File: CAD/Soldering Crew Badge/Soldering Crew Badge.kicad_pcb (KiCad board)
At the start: 2 copper layers, 75.2 x 75.2 mm, 7 parts

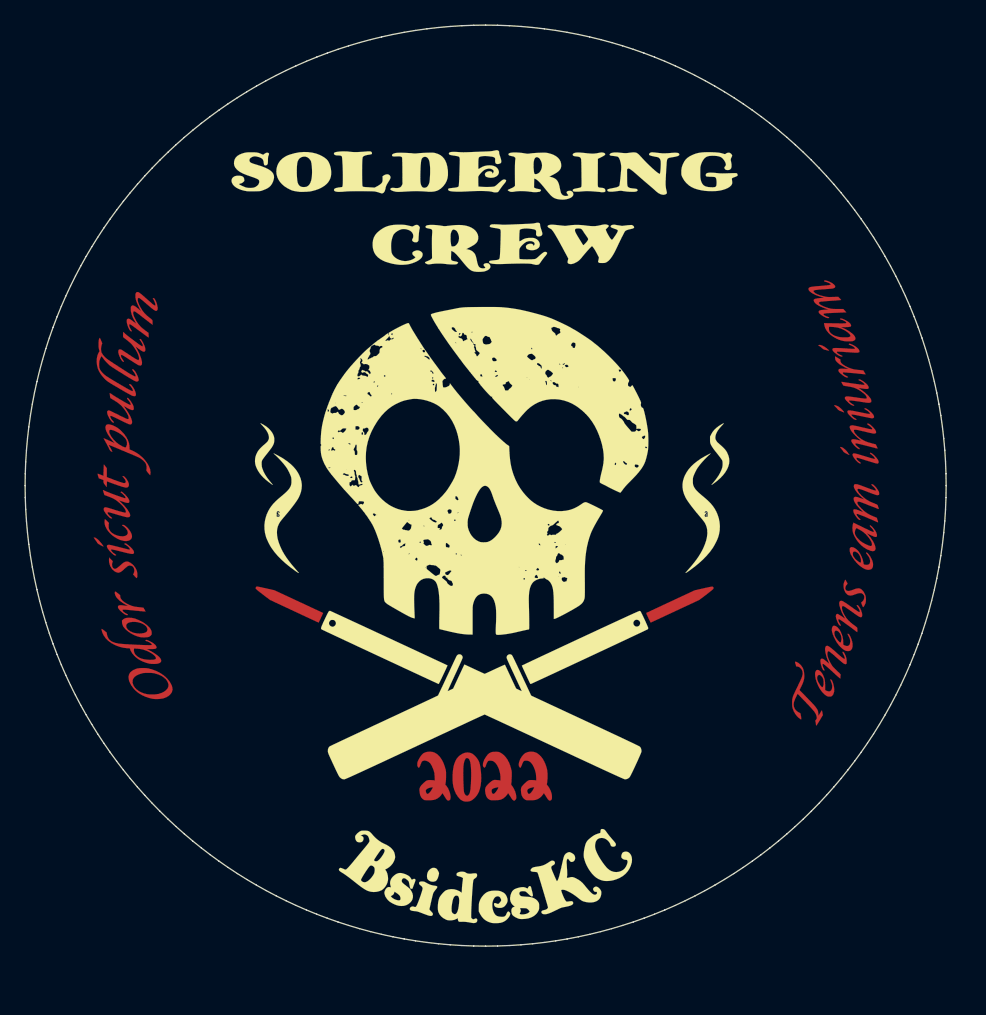
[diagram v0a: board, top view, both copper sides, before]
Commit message: Resized/Updated Soldering Village SAO
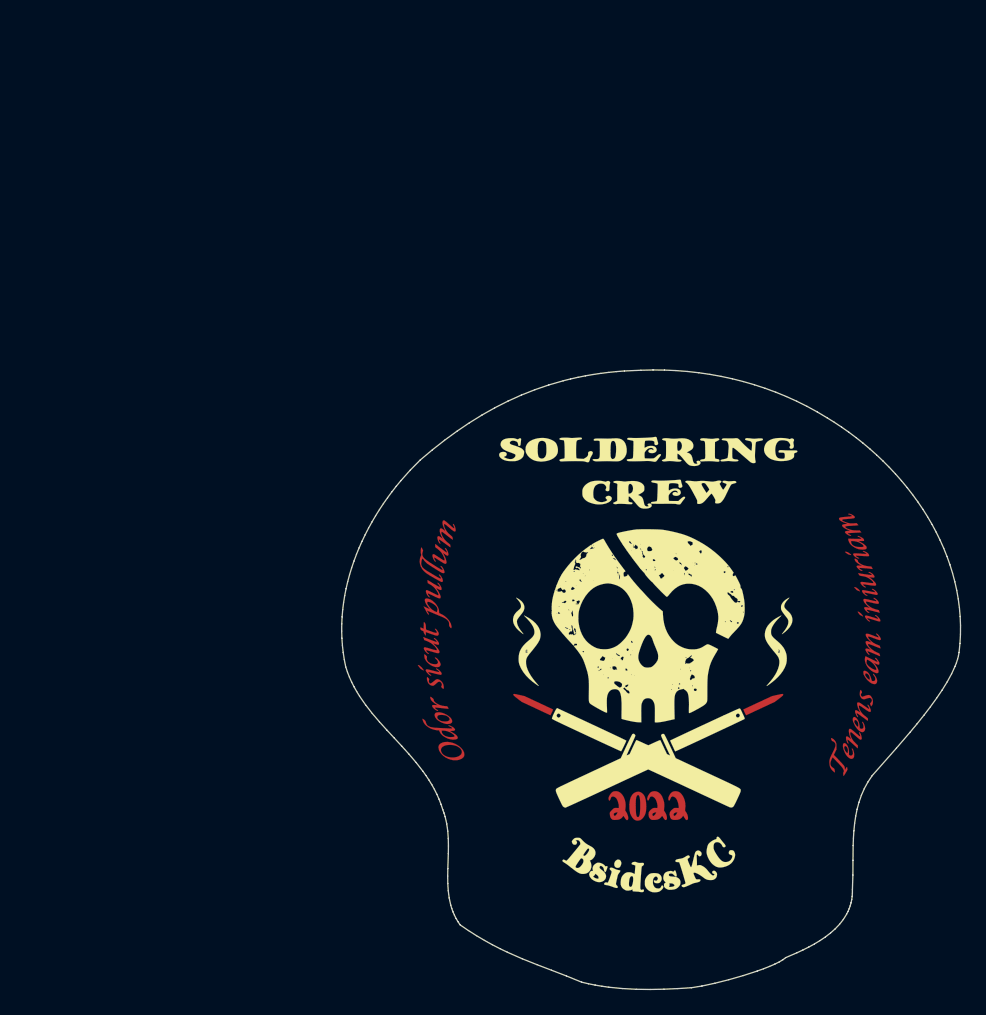
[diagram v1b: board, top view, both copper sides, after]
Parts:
- removed the G*** at (0.00, 0.00) (x7)
- added G*** (x7): LOGO, LOGO, F.Cu at (0.00, 0.00)
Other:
- board size 75.2 x 75.2 mm -> 50.5 x 50.6 mm
